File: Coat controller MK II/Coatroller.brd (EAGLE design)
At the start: 58.4 x 21.6 mm, 11 parts, among them U1 ATMEGA328P_PDIP, U2 V_REG_LDOSMD, Y1 ABM3B-16.000MHZ-B2-T

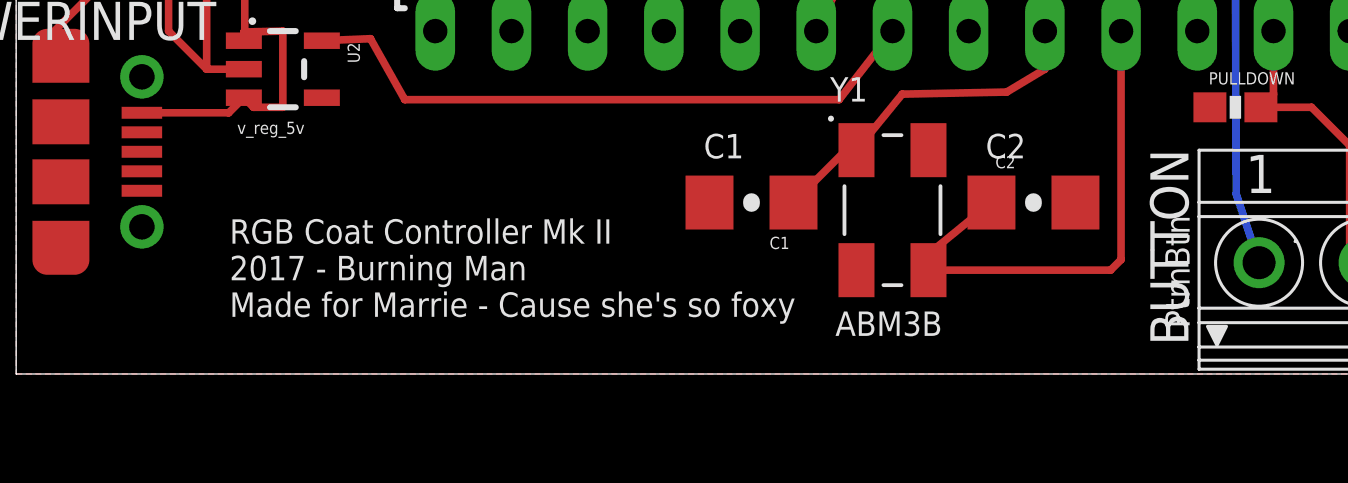
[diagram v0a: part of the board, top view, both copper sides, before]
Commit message: expect this is production level
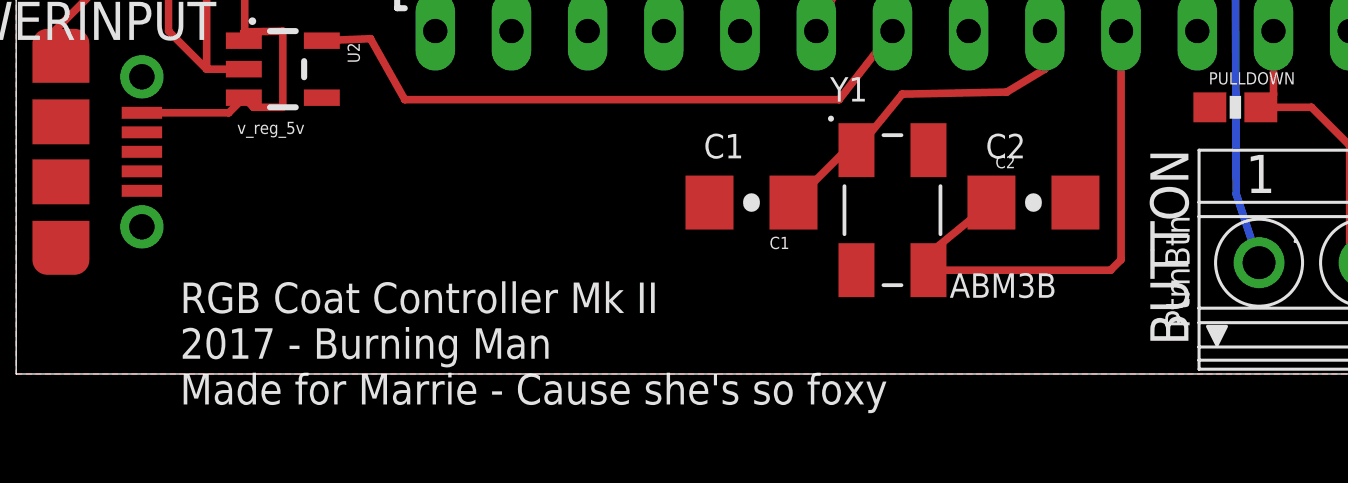
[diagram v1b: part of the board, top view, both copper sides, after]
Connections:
- net GROUND: now also U1.22
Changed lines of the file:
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@@
 <layer number="45" name="Holes" color="7" fill="1" visible="yes" active="yes"/>
 <layer number="46" name="Milling" color="3" fill="1" visible="no" active="yes"/>
-<layer number="47" name="Measures" color="7" fill="1" visible="yes" active="yes"/>
-<layer number="48" name="Document" color="7" fill="1" visible="yes" active="yes"/>
-<layer number="49" name="Reference" color="7" fill="1" visible="yes" active="yes"/>
+<layer number="47" name="Measures" color="7" fill="1" visible="no" active="yes"/>
+<layer number="48" name="Document" color="7" fill="1" visible="no" active="yes"/>
+<layer number="49" name="Reference" color="7" fill="1" visible="no" active="yes"/>
 <layer number="50" name="dxf" color="7" fill="1" visible="no" active="no"/>
 <layer number="51" name="tDocu" color="6" fill="1" visible="yes" active="yes"/>
@@
 <text x="49.149" y="7.874" size="0.8128" layer="21" ratio="15">Clock</text>
 <text x="48.26" y="9.398" size="0.8128" layer="21" ratio="15">Ground</text>
-<text x="27.305" y="1.27" size="0.8128" layer="21" ratio="15">ABM3B</text>
+<text x="31.115" y="2.54" size="0.8128" layer="21" ratio="15">ABM3B</text>
 <text x="24.257" y="8.001" size="0.8128" layer="21" ratio="15" rot="R180">C1</text>
 <text x="8.636" y="14.859" size="0.8128" layer="21" ratio="15" rot="R90">Input</text>
-<text x="7.112" y="1.905" size="0.8128" layer="21" ratio="15">RGB Coat Controller Mk II
+<text x="5.461" y="-1.016" size="1.016" layer="21" ratio="15">RGB Coat Controller Mk II
 2017 - Burning Man
 Made for Marrie - Cause she's so foxy
@@
 <wire x1="6.35" y1="13.97" x2="6.35" y2="10.16" width="0.254" layer="1"/>
 <contactref element="PIN" pad="1"/>
+<contactref element="U1" pad="22"/>
 </signal>
 <signal name="VCC">
